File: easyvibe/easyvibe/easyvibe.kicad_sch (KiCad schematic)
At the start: 87 parts, among them SW1 SW_DPDT_x2, U1 TL062, U2 TL062, U3 TL062, U4 TL062

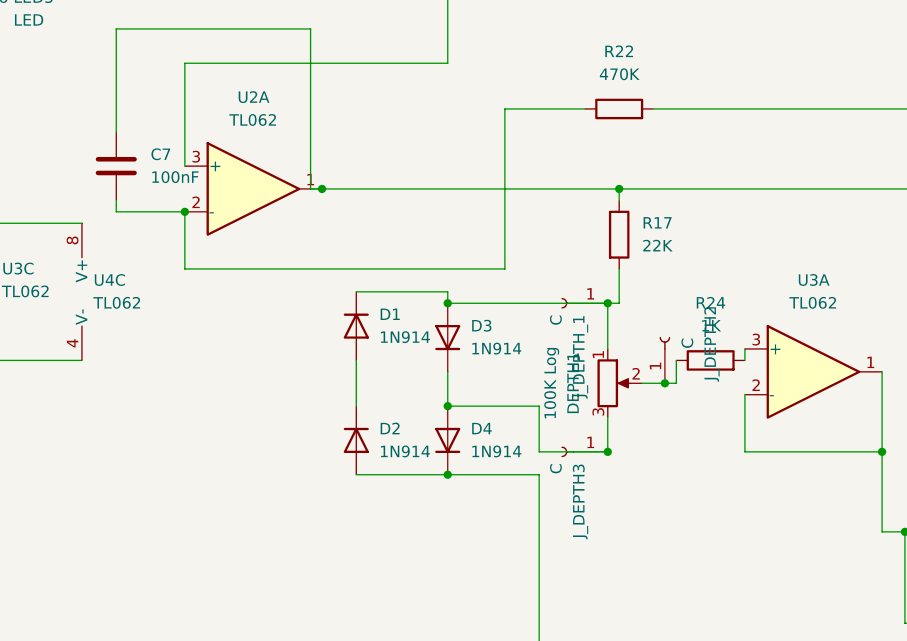
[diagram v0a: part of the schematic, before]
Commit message: more tweaks, make board slightly smaller to fit box
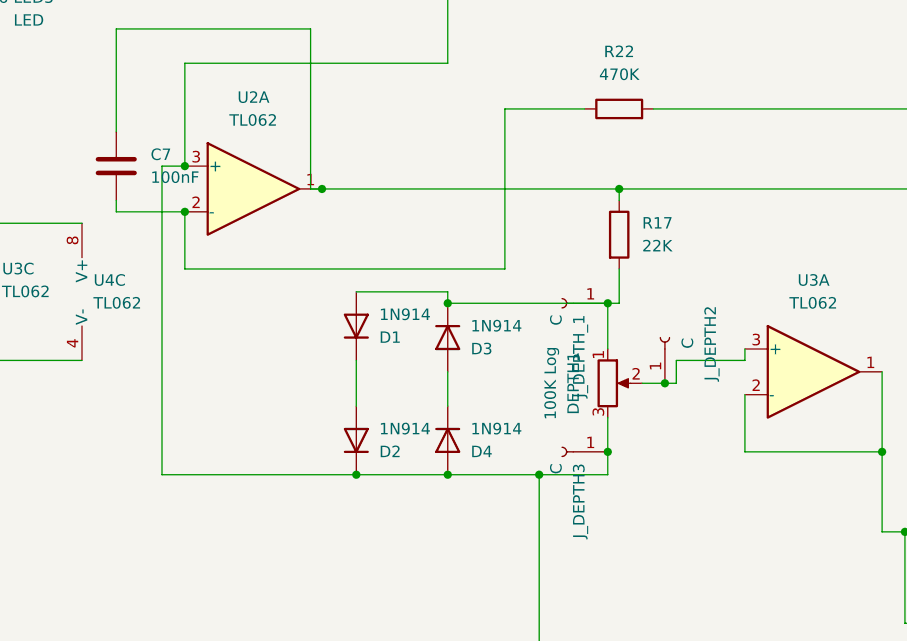
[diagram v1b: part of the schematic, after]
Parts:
- removed R24: 1K, Snapeda:RES_LR1_TYCO_TYC, symbol Device:R
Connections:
- net at R21.2, U4.2 (-): now also C10.1, D2.1 (K), D4.2 (A), D6.2 (A), DEPTH1.3, J_DEPTH3.1 (Pin_1), LDR1.2, LDR2.2, LDR3.2, LDR4.2, R15.2, R2.2, R23.2, R3.2, U2.3 (+); no longer D2.2 (A), D4.1 (K)
- net at DEPTH1.1, J_DEPTH_1.1 (Pin_1), R17.2: now also D1.2 (A), D3.1 (K); no longer D1.1 (K), D3.2 (A)
- net at DEPTH1.2, J_DEPTH2.1 (Pin_1): now also U3.3 (+)
- new net: D3.2 (A), D4.1 (K)
- new net: D1.1 (K), D2.2 (A)
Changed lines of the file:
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@@
 	)
 	(junction
-		(at 106.68 121.92)
-		(diameter 0)
-		(color 0 0 0 0)
-	)
-	(junction
 		(at 179.07 111.76)
 		(diameter 0)
@@
 	)
 	(junction
+		(at 59.69 90.17)
+		(diameter 0)
+		(color 0 0 0 0)
+	)
+	(junction
 		(at 111.76 38.1)
 		(diameter 0)
@@
 	)
 	(junction
-		(at 204.47 38.1)
+		(at 78.74 124.46)
 		(diameter 0)
 		(color 0 0 0 0)
 	)
 	(junction
-		(at 201.93 92.71)
+		(at 106.68 121.92)
 		(diameter 0)
 		(color 0 0 0 0)
 	)
 	(junction
-		(at 127 40.64)
+		(at 204.47 38.1)
 		(diameter 0)
 		(color 0 0 0 0)
 	)
 	(junction
-		(at 88.9 116.84)
+		(at 201.93 92.71)
+		(diameter 0)
+		(color 0 0 0 0)
+	)
+	(junction
+		(at 127 40.64)
 		(diameter 0)
 		(color 0 0 0 0)
@@
 	)
 	(junction
+		(at 99.06 124.46)
+		(diameter 0)
+		(color 0 0 0 0)
+	)
+	(junction
 		(at 105.41 21.59)
 		(diameter 0)
@@
 	(wire
 		(pts
-			(xy 99.06 121.92) (xy 106.68 121.92)
-		)
-		(stroke
-			(width 0)
-			(type default)
-		)
-	)
-	(wire
-		(pts
 			(xy 201.93 148.59) (xy 260.35 148.59)
 		)
@@
 	(wire
 		(pts
+			(xy 59.69 90.17) (xy 57.15 90.17)
+		)
+		(stroke
+			(width 0)
+			(type default)
+		)
+	)
+	(wire
+		(pts
 			(xy 25.4 43.18) (xy 25.4 46.99)
 		)
@@
 	(wire
 		(pts
+			(xy 57.15 90.17) (xy 57.15 124.46)
+		)
+		(stroke
+			(width 0)
+			(type default)
+		)
+	)
+	(wire
+		(pts
 			(xy 63.5 50.8) (xy 63.5 54.61)
 		)
@@
 	(wire
 		(pts
+			(xy 106.68 124.46) (xy 99.06 124.46)
+		)
+		(stroke
+			(width 0)
+			(type default)
+		)
+	)
+	(wire
+		(pts
 			(xy 139.7 140.97) (xy 156.21 140.97)
 		)
@@
 	(wire
 		(pts
-			(xy 99.06 116.84) (xy 99.06 121.92)
-		)
-		(stroke
-			(width 0)
-			(type default)
-		)
-	)
-	(wire
-		(pts
 			(xy 16.51 43.18) (xy 16.51 46.99)
 		)
@@
 	(wire
 		(pts
+			(xy 114.3 111.76) (xy 121.92 111.76)
+		)
+		(stroke
+			(width 0)
+			(type default)
+		)
+	)
+	(wire
+		(pts
 			(xy 81.28 44.45) (xy 81.28 45.72)
 		)
@@
 	(wire
 		(pts
+			(xy 57.15 124.46) (xy 78.74 124.46)
+		)
+		(stroke
+			(width 0)
+			(type default)
+		)
+	)
+	(wire
+		(pts
 			(xy 209.55 46.99) (xy 209.55 48.26)
 		)
@@
 	(wire
 		(pts
-			(xy 88.9 116.84) (xy 99.06 116.84)
-		)
-		(stroke
-			(width 0)
-			(type default)
-		)
-	)
-	(wire
-		(pts
 			(xy 259.08 93.98) (xy 259.08 95.25)
 		)
@@
 	(wire
 		(pts
+			(xy 106.68 121.92) (xy 106.68 124.46)
+		)
+		(stroke
+			(width 0)
+			(type default)
+		)
+	)
+	(wire
+		(pts
 			(xy 184.15 66.04) (xy 189.23 66.04)
 		)
@@
 		(lib_id "Device:D")
 		(at 88.9 120.65 90)
+		(mirror x)
 		(unit 1)
 		(body_style 1)
@@
 		(in_pos_files yes)
 		(dnp no)
-		(fields_autoplaced yes)
 		(property "Reference" "D4"
-			(at 91.44 119.3799 90)
+			(at 91.44 121.9201 90)
 			(show_name no)
 			(do_not_autoplace no)
@@
 		)
 		(property "Value" "1N914"
-			(at 91.44 121.9199 90)
+			(at 91.44 119.3801 90)
 			(show_name no)
 			(do_not_autoplace no)
@@
 		(lib_id "Device:D")
 		(at 78.74 107.95 270)
+		(mirror x)
 		(unit 1)
 		(body_style 1)
@@
 		(in_pos_files yes)
 		(dnp no)
-		(fields_autoplaced yes)
 		(property "Reference" "D1"
-			(at 81.28 106.6799 90)
+			(at 81.28 109.2201 90)
 			(show_name no)
 			(do_not_autoplace no)
@@
 		)
 		(property "Value" "1N914"
-			(at 81.28 109.2199 90)
+			(at 81.28 106.6801 90)
 			(show_name no)
 			(do_not_autoplace no)
@@
 	)
 	(symbol
-		(lib_id "Device:R")
-		(at 118.11 111.76 90)
-		(unit 1)
-		(body_style 1)
-		(exclude_from_sim no)
-		(in_bom yes)
-		(on_board yes)
-		(in_pos_files yes)
-		(dnp no)
-		(fields_autoplaced yes)
-		(property "Reference" "R24"
-			(at 118.11 105.41 90)
-			(show_name no)
-			(do_not_autoplace no)
-			(effects
-				(font
-					(size 1.27 1.27)
-				)
-			)
-		)
-		(property "Value" "1K"
-			(at 118.11 107.95 90)
-			(show_name no)
-			(do_not_autoplace no)
-			(effects
-				(font
-					(size 1.27 1.27)
-				)
-			)
-		)
-		(property "Footprint" "Snapeda:RES_LR1_TYCO_TYC"
-			(at 118.11 113.538 90)
-			(hide yes)
-			(show_name no)
-			(do_not_autoplace no)
-			(effects
-				(font
-					(size 1.27 1.27)
-				)
-			)
-		)
-		(property "Datasheet" ""
-			(at 118.11 111.76 0)
-			(hide yes)
-			(show_name no)
-			(do_not_autoplace no)
-			(effects
-				(font
-					(size 1.27 1.27)
-				)
-			)
-		)
-		(property "Description" "Resistor"
-			(at 118.11 111.76 0)
-			(hide yes)
-			(show_name no)
-			(do_not_autoplace no)
-			(effects
-				(font
-					(size 1.27 1.27)
-				)
-			)
-		)
-		(pin "2"
-		)
-		(pin "1"
-		)
-		(instances
-			(project "easyvibe"
-				(path "/4bb4501e-45c8-4c72-91ca-8621e8761900"
-					(reference "R24")
-					(unit 1)
-				)
-			)
-		)
-	)
-	(symbol
 		(lib_id "Connector:Conn_01x01_Socket")
 		(at 110.49 19.05 90)
@@
 		(lib_id "Device:D")
 		(at 78.74 120.65 270)
+		(mirror x)
 		(unit 1)
 		(body_style 1)
@@
 		(in_pos_files yes)
 		(dnp no)
-		(fields_autoplaced yes)
 		(property "Reference" "D2"
-			(at 81.28 119.3799 90)
+			(at 81.28 121.9201 90)
 			(show_name no)
 			(do_not_autoplace no)
@@
 		)
 		(property "Value" "1N914"
-			(at 81.28 121.9199 90)
+			(at 81.28 119.3801 90)
 			(show_name no)
 			(do_not_autoplace no)
@@
 		(lib_id "Device:D")
 		(at 88.9 109.22 90)
+		(mirror x)
 		(unit 1)
 		(body_style 1)
@@
 		(in_pos_files yes)
 		(dnp no)
-		(fields_autoplaced yes)
 		(property "Reference" "D3"
-			(at 91.44 107.9499 90)
+			(at 91.44 110.4901 90)
 			(show_name no)
 			(do_not_autoplace no)
@@
 		)
 		(property "Value" "1N914"
-			(at 91.44 110.4899 90)
+			(at 91.44 107.9501 90)
 			(show_name no)
 			(do_not_autoplace no)
